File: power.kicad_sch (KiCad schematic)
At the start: 21 parts, among them U3 LM66200DRLR, U4 SC4215, U5 MAX77827AEFD+T

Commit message: Add photo triggers
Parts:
- U3: footprint iclr:SOTFL50P160X60-8N -> fps:SOTFL50P160X60-8N
- U4: footprint iclr:SOIC127P599X175-9N -> fps:SOIC127P599X175-8N
- U5: footprint iclr:CONV_MAX77827AEFD+T -> fps:CONV_MAX77827AEFD+T
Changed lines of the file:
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@@
       (effects (font (size 1.27 1.27)))
     )
-    (property "Footprint" "iclr:SOTFL50P160X60-8N" (at 76.2 34.29 0)
+    (property "Footprint" "fps:SOTFL50P160X60-8N" (at 76.2 34.29 0)
       (effects (font (size 1.27 1.27)) (justify left) hide)
     )
@@
       (effects (font (size 1.27 1.27)))
     )
-    (property "Footprint" "iclr:SOIC127P599X175-9N" (at 218.44 45.72 0)
+    (property "Footprint" "fps:SOIC127P599X175-8N" (at 218.44 45.72 0)
       (effects (font (size 1.27 1.27)) hide)
     )
@@
       (effects (font (size 1.27 1.27)))
     )
-    (property "Footprint" "iclr:CONV_MAX77827AEFD+T" (at 144.78 43.18 0)
+    (property "Footprint" "fps:CONV_MAX77827AEFD+T" (at 144.78 43.18 0)
       (effects (font (size 1.27 1.27)) (justify left bottom) hide)
     )

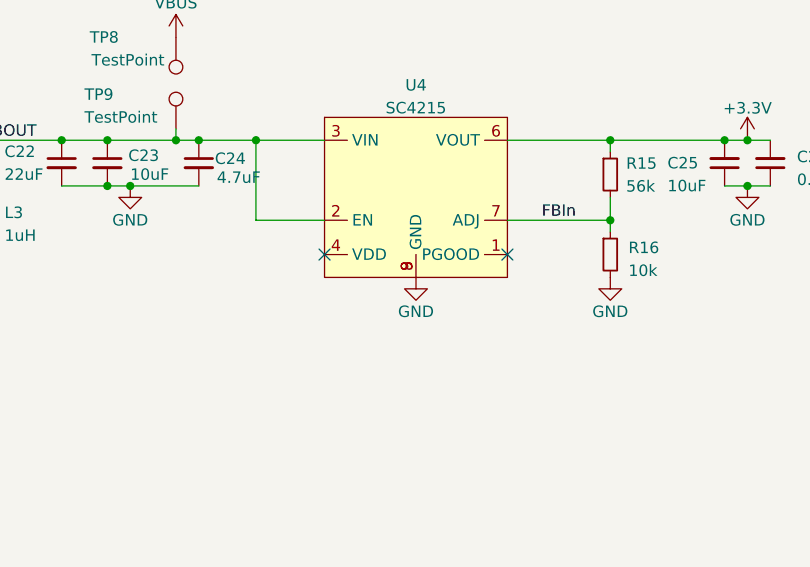
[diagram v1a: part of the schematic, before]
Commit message: Fixed libraries and footprints
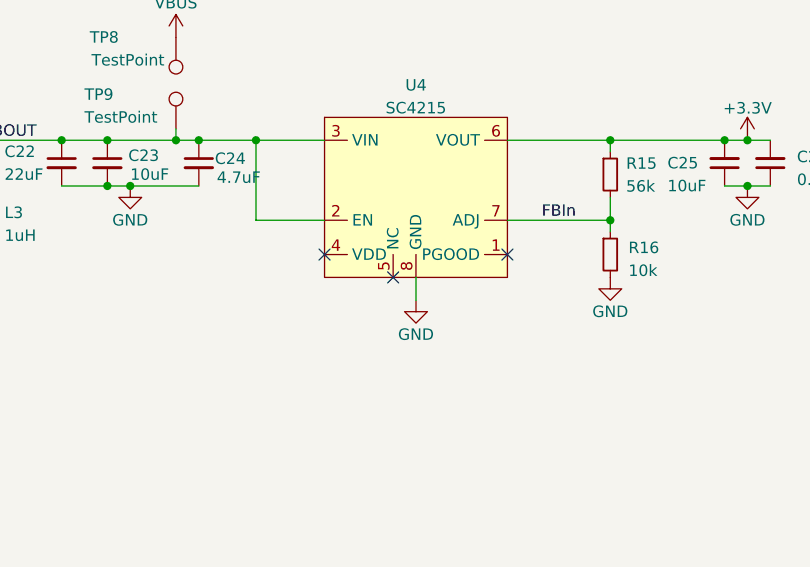
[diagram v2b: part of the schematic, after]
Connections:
- net GND: no longer U4.9 (GND)
- no-connect marks 4 -> 5
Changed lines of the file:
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@@
   (junction (at 200.66 52.07) (diameter 0) (color 0 0 0 0)
   )
+  (no_connect (at 215.9 67.31))
   (no_connect (at 166.37 67.31))
   (no_connect (at 135.89 59.69))
@@
   )
   (wire (pts (xy 240.03 60.96) (xy 240.03 62.23))
+    (stroke (width 0) (type default))
+  )
+  (wire (pts (xy 218.44 67.31) (xy 218.44 69.85))
     (stroke (width 0) (type default))
   )
@@
     )
   )
-  (symbol (lib_id "power:GND") (at 218.44 67.31 0) (unit 1)
-    (in_bom yes) (on_board yes) (dnp no)
-    (property "Reference" "#PWR047" (at 218.44 73.66 0)
-      (effects (font (size 1.27 1.27)) hide)
-    )
-    (property "Value" "GND" (at 218.44 71.12 0)
-      (effects (font (size 1.27 1.27)))
-    )
-    (property "Footprint" "" (at 218.44 67.31 0)
-      (effects (font (size 1.27 1.27)) hide)
-    )
-    (property "Datasheet" "" (at 218.44 67.31 0)
+  (symbol (lib_id "power:GND") (at 218.44 69.85 0) (unit 1)
+    (in_bom yes) (on_board yes) (dnp no)
+    (property "Reference" "#PWR047" (at 218.44 76.2 0)
+      (effects (font (size 1.27 1.27)) hide)
+    )
+    (property "Value" "GND" (at 218.44 73.66 0)
+      (effects (font (size 1.27 1.27)))
+    )
+    (property "Footprint" "" (at 218.44 69.85 0)
+      (effects (font (size 1.27 1.27)) hide)
+    )
+    (property "Datasheet" "" (at 218.44 69.85 0)
       (effects (font (size 1.27 1.27)) hide)
     )
@@
     (pin "3")
     (pin "4")
+    (pin "5")
     (pin "6")
     (pin "7")
     (pin "8")
-    (pin "9")
-    (instances
-      (project "RicardoCHEESE"
+    (instances
+      (project "RicardoCHEESE"
